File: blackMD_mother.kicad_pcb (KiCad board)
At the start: 2 copper layers, 99.1 x 99.1 mm, 19 parts

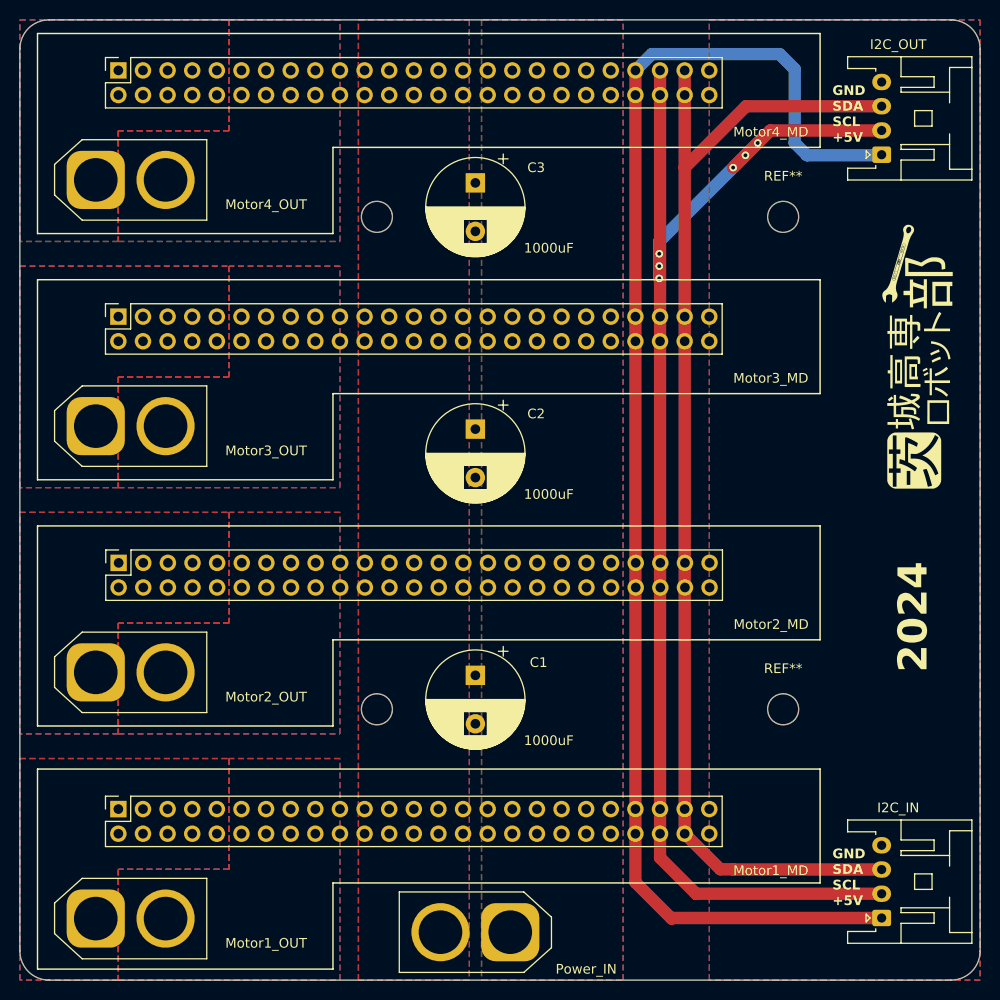
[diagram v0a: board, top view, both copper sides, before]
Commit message: change: width of GNDPWR
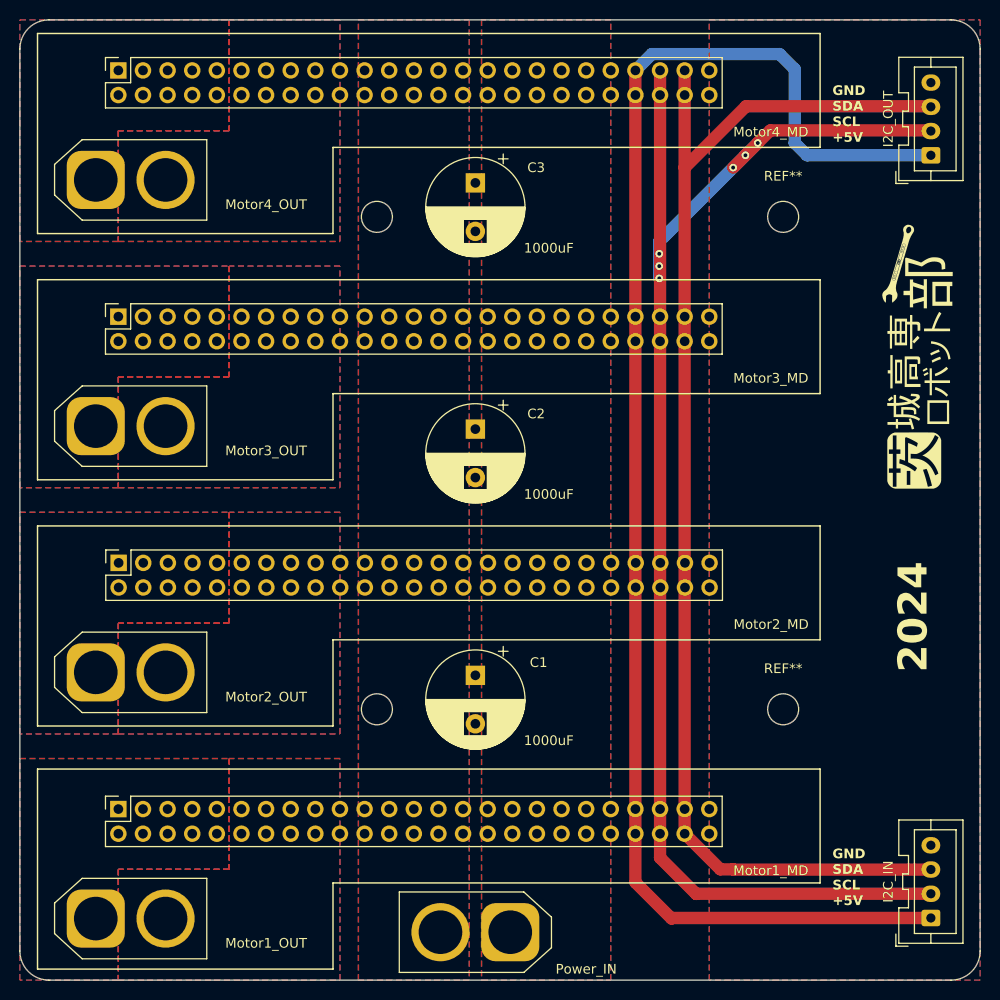
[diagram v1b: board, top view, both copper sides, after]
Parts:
- I2C_IN, I2C_OUT: footprint Connector_JST:JST_XA_S04B-XASK-1_1x04_P2.50mm_Horizontal -> Connector_JST:JST_XA_B04B-XASK-1_1x04_P2.50mm_Vertical
- moved I2C_OUT 5.08 mm to (186.8, 68.6)
- moved I2C_IN 5.08 mm to (186.8, 147.3)
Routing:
- net SDA: track 123.5 -> 133.7 mm
- net SCL: track 140.7 -> 150.9 mm
- net +5V: track 145.6 -> 155.8 mm

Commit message: Revert "change: width of GNDPWR"
This reverts commit 1e5340b1a1ce9a68678be1db281a547735c12933.
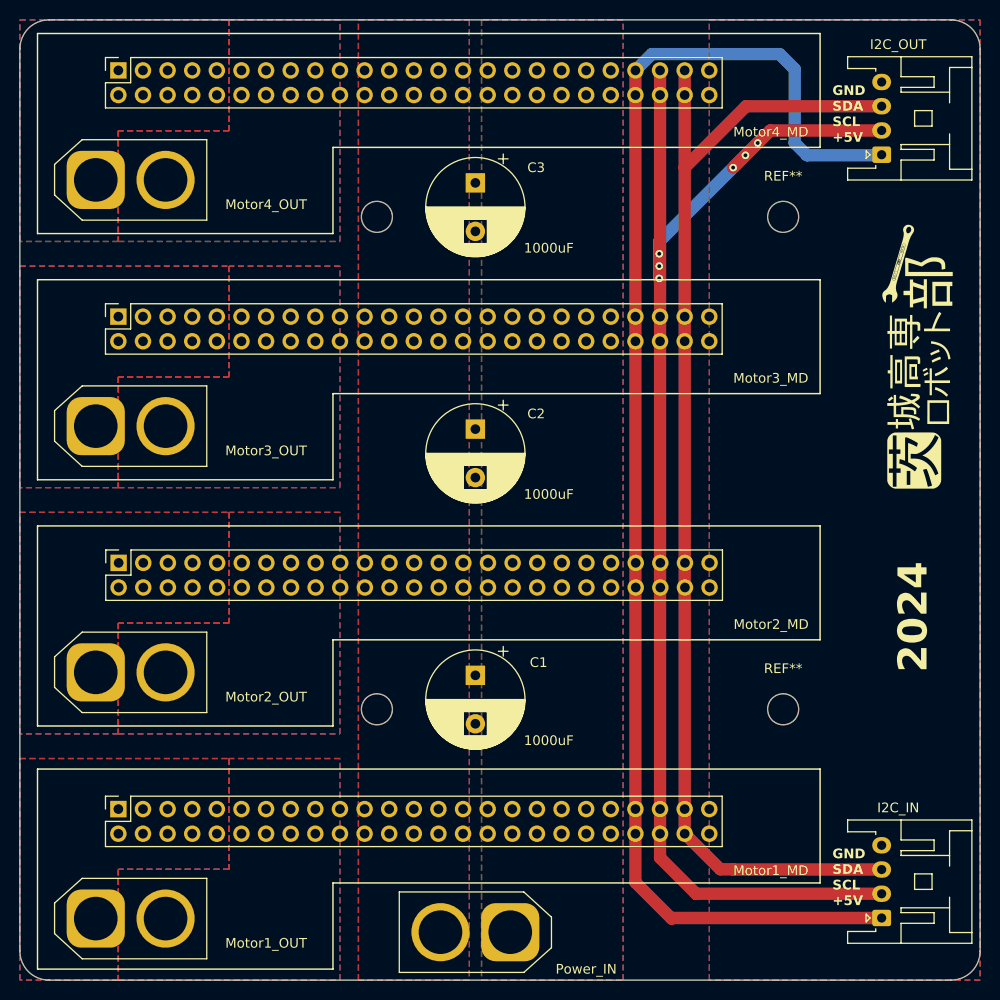
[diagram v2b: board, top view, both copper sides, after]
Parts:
- I2C_IN, I2C_OUT: footprint Connector_JST:JST_XA_B04B-XASK-1_1x04_P2.50mm_Vertical -> Connector_JST:JST_XA_S04B-XASK-1_1x04_P2.50mm_Horizontal
- moved I2C_OUT 5.08 mm to (181.7, 68.5)
- moved I2C_IN 5.08 mm to (181.7, 147.3)
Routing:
- net SDA: track 133.7 -> 123.5 mm
- net SCL: track 150.9 -> 140.7 mm
- net +5V: track 155.8 -> 145.6 mm
